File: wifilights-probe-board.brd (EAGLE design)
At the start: 50.8 x 50.8 mm, 48 parts, among them Q1 BUK98180-100A, Q2 BUK98180-100A, Q3 BUK98180-100A, Q4 BUK98180-100A, U2 PCA9685

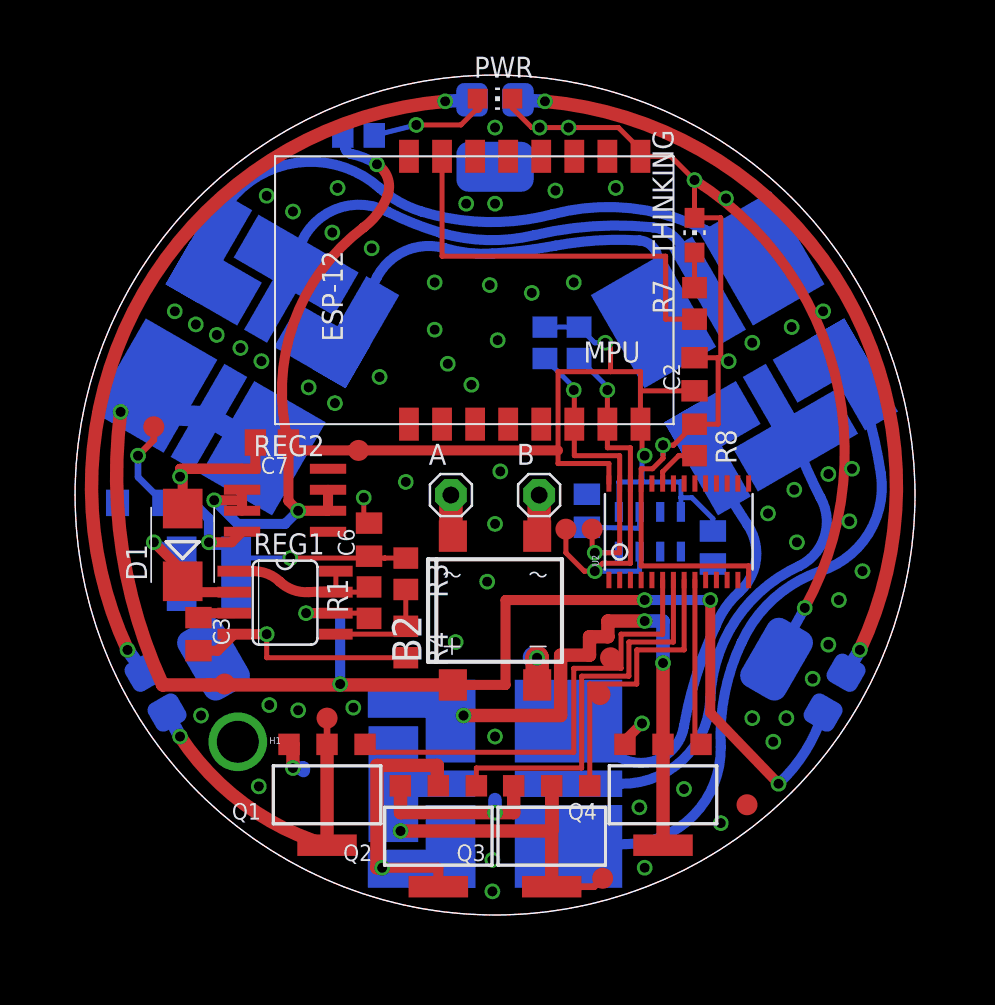
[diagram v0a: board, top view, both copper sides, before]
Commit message: Probe board complete
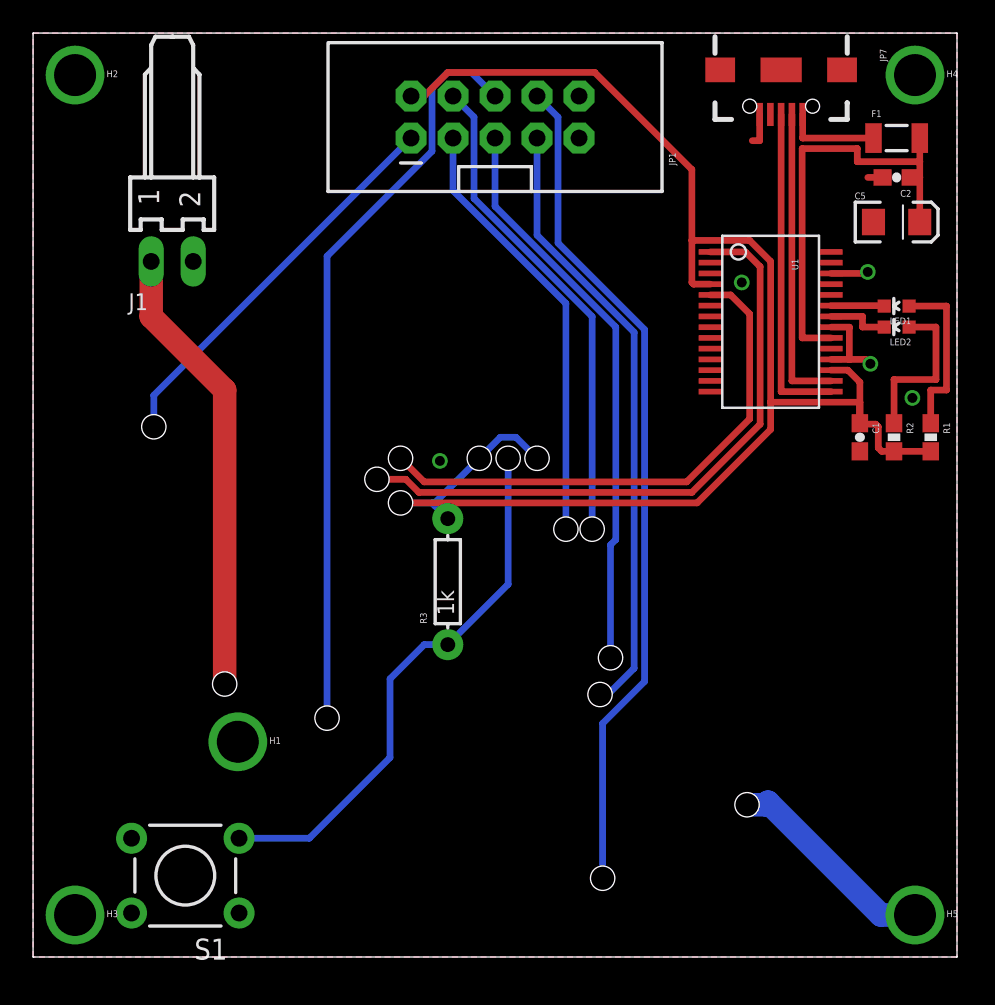
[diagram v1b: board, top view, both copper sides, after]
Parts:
- removed A, B: (no value), adafruit:1X01
- removed B2: DBLS203G, rectifier:DBS
- removed C3: 220pf, resistor:C0805K
- removed C4, C6: 0.1uF, resistor:C0805K
- removed C7: 10uF, resistor:C0805K
- removed D1: MBRS140T3, diode:SMB
- removed L1: 220uf, SparkFun-Passives:SDR0403
- removed LED3: OVSTRGBBCR8, led:OVSTRGBBCR8
- removed MPU: ESP8266_ESP-12, ESP8266-ESP12:ESP8266-ESP12
- removed PWR, THINKING: (no value), led:CHIP-LED0805
- removed Q1, Q2, Q3, Q4: BUK98180-100A, nxp_60:SOT223
- removed R4: 1K, resistor:R0805
- removed R5, R6: 1k, resistor:R0805
- removed R7: ???, resistor:R0805
- removed R8: 10K, resistor:R0805
- removed REG1: MC33063/MC34063D, adafruit:SO08
- removed REG2: MC33269-SO8, linear:SO08
- removed TEMPERATURE: MPL3115A2LGA8, SparkFun-Sensors:LGA8
- removed U$1, U$2, U$3: LUXEON-REBEL, SparkFun-LED:LUXEON-REBEL
- removed U2: PCA9685, adafruit:TSSOP28
- added F1: 500mA, SparkFun:PTC-1206
- added H2, H3, H4, H5: SEW_HOLE, LilyPad-Wearables:SIMPLE_HOLE
- added J1: 22-05-7028-02, con-molex:7395-02
- added JP1: (no value), SparkFun-Connectors:2X5-SHROUDED
- added JP7: USB_MICROB_PLUGCONN-11752, SparkFun-Connectors:USB-B-MICRO-SMD_V03
- added S1: SWITCH-MOMENTARY-2PTH, SparkFun-Electromechanical:TACTILE-PTH
- added TPCHPD, TPGPIO0, TPGPIO2, TPRX, TPTX: (no value), SparkFun-Connectors:1X01_POGOPIN_HOLE_0.58
- added U1: FT232R, SparkFun:SSOP28DB
- C1, C2: device resistor:C0805K -> SparkFun-Capacitors:0603-CAP
- LED1: value OVSTRGBBCR8 -> Red; device led:OVSTRGBBCR8 -> SparkFun-LED:LED-0603
- LED2: value OVSTRGBBCR8 -> Green; device led:OVSTRGBBCR8 -> SparkFun-LED:LED-0603
- P_RED, P_WHITE, RED, SCL, SDA, TP12V, TP3.3V, TP5V, TPGND, WHITE: value TEST-POINT3X5 -> (none); device SparkFun-Passives:PAD.03X.05 -> SparkFun-Connectors:1X01_POGOPIN_HOLE_0.58
- R1: value 220 ??? -> 330; device resistor:R0805 -> SparkFun-Resistors:0603-RES
- R2: value ??? -> 330; device resistor:R0805 -> SparkFun-Resistors:0603-RES
- R3: value 3K -> 1k; device resistor:R0805 -> SparkFun-Passives:AXIAL-0.3
- moved C5 48.8 mm to (49.7, 41.9), flipped to the top, turned to 0 degrees
- moved LED1 39.5 mm to (49.7, 36.8), flipped to the top, turned to 90 degrees
- moved R2 37.2 mm to (49.5, 28.9), flipped to the top, turned to 270 degrees
- moved R1 35.4 mm to (51.8, 28.9), turned to 270 degrees
- moved C2 17.1 mm to (49.7, 44.6), turned to 180 degrees
- moved C1 11.1 mm to (47.5, 28.9), flipped to the top
- moved LED2 9.34 mm to (49.7, 35.6), flipped to the top, turned to 90 degrees
- moved TP3.3V 4.07 mm to (19.7, 24.9)
- moved R3 2.58 mm to (22.5, 20.2), turned to 90 degrees
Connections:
- removed net BLUE: Q2.1, U2.7
- removed net COMP: R3.2, R4.1, REG1.5
- removed net GREEN: Q4.1, U2.9
- removed net N$10: U$1.CATHODE, U$2.ANODE
- removed net N$11: U$2.CATHODE, U$3.ANODE
- removed net N$13: R1.2, REG1.1, REG1.7, REG1.8
- removed net N$14: PWR.A, R2.2
- removed net N$15: R7.2, THINKING.A
- removed net N$16: C3.1, REG1.3
- removed net N$17: C4.1, TEMPERATURE.2
- removed net N$18: A.1, B2.AC1
- removed net N$19: B.1, B2.AC2
- removed net N$20: R8.2, U2.23
- removed net N$25: MPU.13
- removed net N$26: MPU.12
- removed net N$27: MPU.11
- removed net N$28: MPU.10
- removed net N$29: MPU.9
- removed net N$32: MPU.6
- removed net N$33: MPU.4
- removed net N$34: MPU.3
- removed net N$35: MPU.2
- removed net N$36: MPU.5
- removed net N$5: LED2.5, LED2.5@1, LED3.2
- removed net N$6: LED1.5, LED1.5@1, LED2.2
- removed net N$7: LED1.6, LED1.6@1, LED2.3
- removed net N$8: LED2.6, LED2.6@1, LED3.3
- removed net P_BLUE: LED3.6, LED3.6@1, Q2.2, Q2.4
- removed net P_GREEN: LED3.4, LED3.4@1, Q4.2, Q4.4
- removed net RESET: MPU.8
- removed net SWE: D1.C, L1.P$2, REG1.2
- removed net THINKING: MPU.7, R7.1
- new net CTS: U1.11
- new net DCD: U1.10
- new net DSR: U1.9
- new net DTR: U1.2
- new net GPIO0: R3.P$1, S1.3, TPGPIO0.1
- new net N$3: F1.1, JP7.VBUS1
- new net PWREN: U1.14
- new net RI: U1.6
- new net RTS: U1.3
- new net RXD: TPRX.1, U1.5
- new net RXLED: LED2.C, U1.22
- new net SLEEP: U1.12
- new net TXD: TPTX.1, U1.1
- new net TXDEN: U1.13
- new net TXLED: LED1.C, U1.23
- new net USB_D+: JP7.D+1, U1.15
- new net USB_D-: JP7.D-1, U1.16
- new net VCC: C2.1, C5.A, F1.2, U1.20
- net 12V: now also J1.1, TP12V.1; no longer B2.+, LED1.1, LED1.2, LED1.3, R1.1, REG1.6, TP12V.P$1, U$1.ANODE
- net 3.3V: now also JP1.2, R1.2, R2.2, R3.P$2, TP3.3V.1, TPCHPD.1, TPGPIO2.1, U1.17, U1.4; no longer C2.1, C7.1, MPU.16, R2.1, R5.2, R6.2, REG2.2, REG2.3, REG2.6, REG2.7, TEMPERATURE.1, TEMPERATURE.4, TP3.3V.P$1, U2.28
- net 5V: now also JP1.1, TP5V.1; no longer C5.A, C6.1, L1.P$1, R3.1, REG2.4, TP5V.P$1
- net GND: now also H2.P$1, H3.P$1, H4.P$1, H5.P$1, J1.2, JP1.10, JP1.9, JP7.GND1, S1.1, TPGND.1, U1.18, U1.21, U1.25, U1.26, U1.7; no longer B2.-, C3.2, C4.2, C6.2, C7.2, D1.A, MPU.1, PWR.C, Q1.3, Q2.3, Q3.3, Q4.3, R4.2, R8.1, REG1.4, REG2.1, TEMPERATURE.3, THINKING.C, TPGND.P$1, U$1.P$3, U$2.P$3, U$3.P$3, U2.14, U2.25
- net N$1: now also LED1.A, R1.1; no longer LED1.4, LED1.4@1, LED2.1
- net N$2: now also LED2.A, R2.1; no longer LED2.4, LED2.4@1, LED3.1
- net P_RED: now also JP1.8, P_RED.1; no longer LED3.5, LED3.5@1, P_RED.P$1, Q3.2, Q3.4
- net P_WHITE: now also JP1.6, P_WHITE.1; no longer P_WHITE.P$1, Q1.2, Q1.4, U$3.CATHODE
- net RED: now also JP1.7, RED.1; no longer Q3.1, RED.P$1, U2.8
- net SCL: now also JP1.3, SCL.1; no longer MPU.15, R6.1, SCL.P$1, TEMPERATURE.7, U2.26
- net SDA: now also JP1.4, SDA.1; no longer MPU.14, R5.1, SDA.P$1, TEMPERATURE.8, U2.27
- net WHITE: now also JP1.5, WHITE.1; no longer Q1.1, U2.6, WHITE.P$1
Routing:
- net GND: track 128.2 -> 23.8 mm, vias 73 -> 5
- net 12V: track 111.5 -> 27.4 mm, vias 6 -> 0
- net N$11: track 41.7 -> 0.00 mm, vias 2 -> 0
- net N$10: track 41.5 -> 0.00 mm, vias 2 -> 0
- net TXD: track 0.00 -> 38.1 mm
- net N$8: track 37.7 -> 0.00 mm
- net N$7: track 34.9 -> 0.00 mm
- net P_GREEN: track 34.1 -> 0.00 mm, vias 3 -> 0
- net GPIO0: track 0.00 -> 33.0 mm
- net RXD: track 0.00 -> 32.5 mm
- net N$5: track 28.4 -> 0.00 mm
- net N$6: track 27.9 -> 0.00 mm
- net VCC: track 0.00 -> 26.7 mm
- net P_RED: track 24.5 -> 51.1 mm, vias 1 -> 0
- net P_WHITE: track 20.4 -> 45.5 mm, vias 1 -> 0
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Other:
- board size 50.8 x 50.8 mm -> 55.9 x 55.9 mm
